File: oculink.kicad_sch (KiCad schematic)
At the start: 17 parts, among them J4 OCuLink_x4_Amphenol_G14A42121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, U10 ESD204DQAR, U11 ESD204DQAR, U8 ESD204DQAR, U9 ESD204DQAR

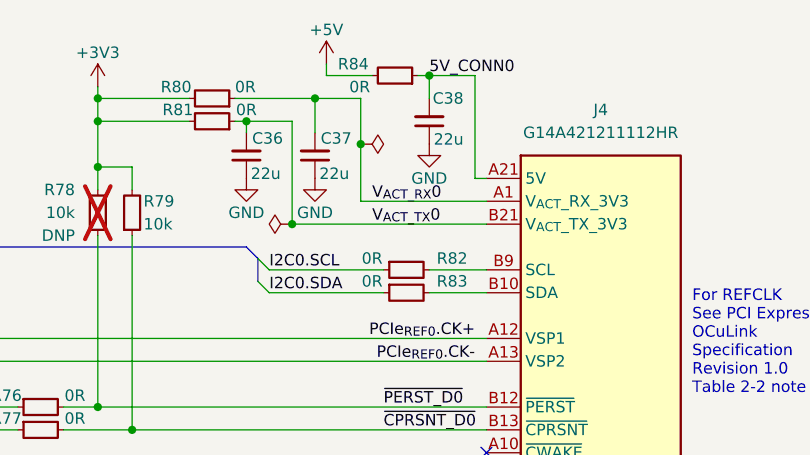
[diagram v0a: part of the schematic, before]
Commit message: Optimize BOM, reannotate
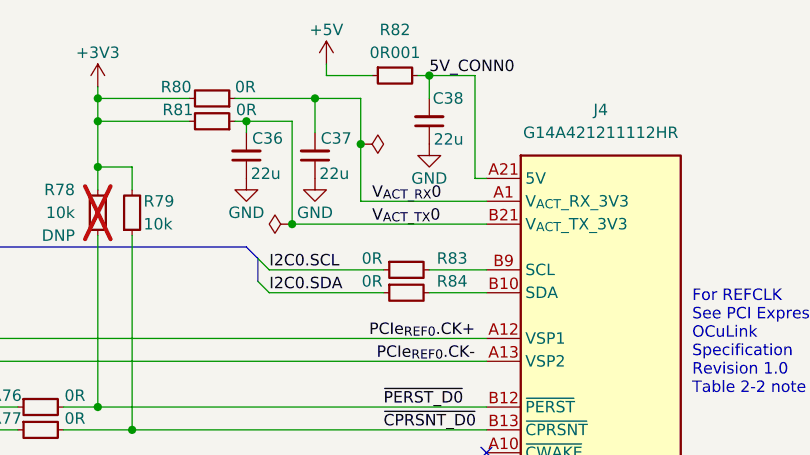
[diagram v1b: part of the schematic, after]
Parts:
- removed R84: R_0R_0603, antmicro-footprints:R_0603_1608Metric, symbol antmicroResistors0603:R_0R_0603
- added R82: R_0R001_0805, antmicro-footprints:R_0805_2012Metric, symbol antmicroResistorsmisc:R_0R001_0805
- renumbered R82 to R83, R83 to R84
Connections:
- net +5V: now also R82.1
- net 5V_CONN0: now also R82.2
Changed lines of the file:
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@@
+    )
+  )
+  (symbol (lib_id "antmicroResistorsmisc:R_0R001_0805") (at 224.79 87.63 0) (unit 1)
+    (in_bom yes) (on_board yes) (dnp no)
+    (property "Reference" "R82" (at 227.33 82.55 0)
+      (effects (font (size 1.27 1.27) (thickness 0.15)))
+    )
+    (property "Value" "R_0R001_0805" (at 245.11 100.33 0)
+      (effects (font (size 1.27 1.27) (thickness 0.15)) (justify left bottom) hide)
+    )
+    (property "Footprint" "antmicro-footprints:R_0805_2012Metric" (at 245.11 102.87 0)
+      (effects (font (size 1.27 1.27) (thickness 0.15)) (justify left bottom) hide)
+    )
+    (property "Datasheet" "https://www.bourns.com/docs/product-datasheets/cr.pdf" (at 245.11 105.41 0)
+      (effects (font (size 1.27 1.27) (thickness 0.15)) (justify left bottom) hide)
+    )
+    (property "MPN" "MSMA0805R0010FSM" (at 245.11 107.95 0)
+      (effects (font (size 1.27 1.27) (thickness 0.15)) (justify left bottom) hide)
+    )
+    (property "Manufacturer" "Eaton" (at 245.11 110.49 0)
+      (effects (font (size 1.27 1.27) (thickness 0.15)) (justify left bottom) hide)
+    )
+    (property "License" "Apache-2.0" (at 245.11 113.03 0)
+      (effects (font (size 1.27 1.27) (thickness 0.15)) (justify left bottom) hide)
+    )
+    (property "Author" "Antmicro" (at 245.11 115.57 0)
+      (effects (font (size 1.27 1.27) (thickness 0.15)) (justify left bottom) hide)
+    )
+    (property "Val" "0R001" (at 227.33 85.09 0)
+      (effects (font (size 1.27 1.27) (thickness 0.15)))
+    )
+    (property "Tolerance" "1%" (at 245.11 97.79 0)
+      (effects (font (size 1.27 1.27)) (justify left bottom) hide)
+    )
+    (pin "2")
+    (pin "1")
+    (instances
+      (project "com-express-7-baseboard"
+        (path "/1b8c34da-dad5-4b0b-8c4b-45db766c4dfa/b09f3a23-0194-4388-b358-3a9807b09321"
+          (reference "R82") (unit 1)
+        )
+      )
     )
   )
@@
     )
   )
-  (symbol (lib_id "antmicroResistors0603:R_0R_0603") (at 229.87 87.63 180) (unit 1)
-    (in_bom yes) (on_board yes) (dnp no)
-    (property "Reference" "R84" (at 220.98 86.36 0)
-      (effects (font (size 1.27 1.27) (thickness 0.15)) (justify right))
-    )
-    (property "Value" "R_0R_0603" (at 209.55 74.93 0)
-      (effects (font (size 1.27 1.27) (thickness 0.15)) (justify left bottom) hide)
-    )
-    (property "Footprint" "antmicro-footprints:R_0603_1608Metric" (at 209.55 72.39 0)
-      (effects (font (size 1.27 1.27) (thickness 0.15)) (justify left bottom) hide)
-    )
-    (property "Datasheet" "https://www.bourns.com/docs/product-datasheets/cr.pdf?sfvrsn=574d41f6_14" (at 209.55 69.85 0)
-      (effects (font (size 1.27 1.27) (thickness 0.15)) (justify left bottom) hide)
-    )
-    (property "MPN" "CR0603-J/-000ELF" (at 209.55 67.31 0)
-      (effects (font (size 1.27 1.27) (thickness 0.15)) (justify left bottom) hide)
-    )
-    (property "Manufacturer" "Bourns" (at 209.55 64.77 0)
-      (effects (font (size 1.27 1.27) (thickness 0.15)) (justify left bottom) hide)
-    )
-    (property "License" "Apache-2.0" (at 209.55 62.23 0)
-      (effects (font (size 1.27 1.27) (thickness 0.15)) (justify left bottom) hide)
-    )
-    (property "Author" "Antmicro" (at 209.55 59.69 0)
-      (effects (font (size 1.27 1.27) (thickness 0.15)) (justify left bottom) hide)
-    )
-    (property "Val" "0R" (at 222.25 88.9 0)
-      (effects (font (size 1.27 1.27) (thickness 0.15)) (justify right))
-    )
-    (property "Tolerance" "~" (at 209.55 77.47 0)
-      (effects (font (size 1.27 1.27)) (justify left bottom) hide)
-    )
-    (property "Current" "1A" (at 209.55 57.15 0)
-      (effects (font (size 1.27 1.27) (thickness 0.15)) (justify left bottom) hide)
-    )
-    (pin "2")
-    (pin "1")
-    (instances
-      (project "com-express-7-baseboard"
-        (path "/1b8c34da-dad5-4b0b-8c4b-45db766c4dfa/b09f3a23-0194-4388-b358-3a9807b09321"
-          (reference "R84") (unit 1)
-        )
-      )
-    )
-  )
   (symbol (lib_id "antmicropower:+3V3") (at 194.31 88.9 0) (unit 1)
     (in_bom yes) (on_board yes) (dnp no)
@@
   (symbol (lib_id "antmicroResistors0402:R_0R_0402") (at 226.06 109.22 0) (unit 1)
     (in_bom yes) (on_board yes) (dnp no)
-    (property "Reference" "R82" (at 233.68 107.95 0)
+    (property "Reference" "R83" (at 233.68 107.95 0)
       (effects (font (size 1.27 1.27) (thickness 0.15)))
     )
@@
       (project "com-express-7-baseboard"
         (path "/1b8c34da-dad5-4b0b-8c4b-45db766c4dfa/b09f3a23-0194-4388-b358-3a9807b09321"
-          (reference "R82") (unit 1)
+          (reference "R83") (unit 1)
         )
       )
@@
   (symbol (lib_id "antmicroResistors0402:R_0R_0402") (at 226.06 111.76 0) (unit 1)
     (in_bom yes) (on_board yes) (dnp no)
-    (property "Reference" "R83" (at 233.68 110.49 0)
+    (property "Reference" "R84" (at 233.68 110.49 0)
       (effects (font (size 1.27 1.27) (thickness 0.15)))
     )
@@
       (project "com-express-7-baseboard"
         (path "/1b8c34da-dad5-4b0b-8c4b-45db766c4dfa/b09f3a23-0194-4388-b358-3a9807b09321"
-          (reference "R83") (unit 1)
-        )
-      )
+          (reference "R84") (unit 1)
+        )
+      )
